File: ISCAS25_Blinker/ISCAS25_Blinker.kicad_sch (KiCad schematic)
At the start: 18 parts, among them J1 USB_C_Receptacle_PowerOnly_6P, Q1 BC846, Q2 BC857, U2 NE555D

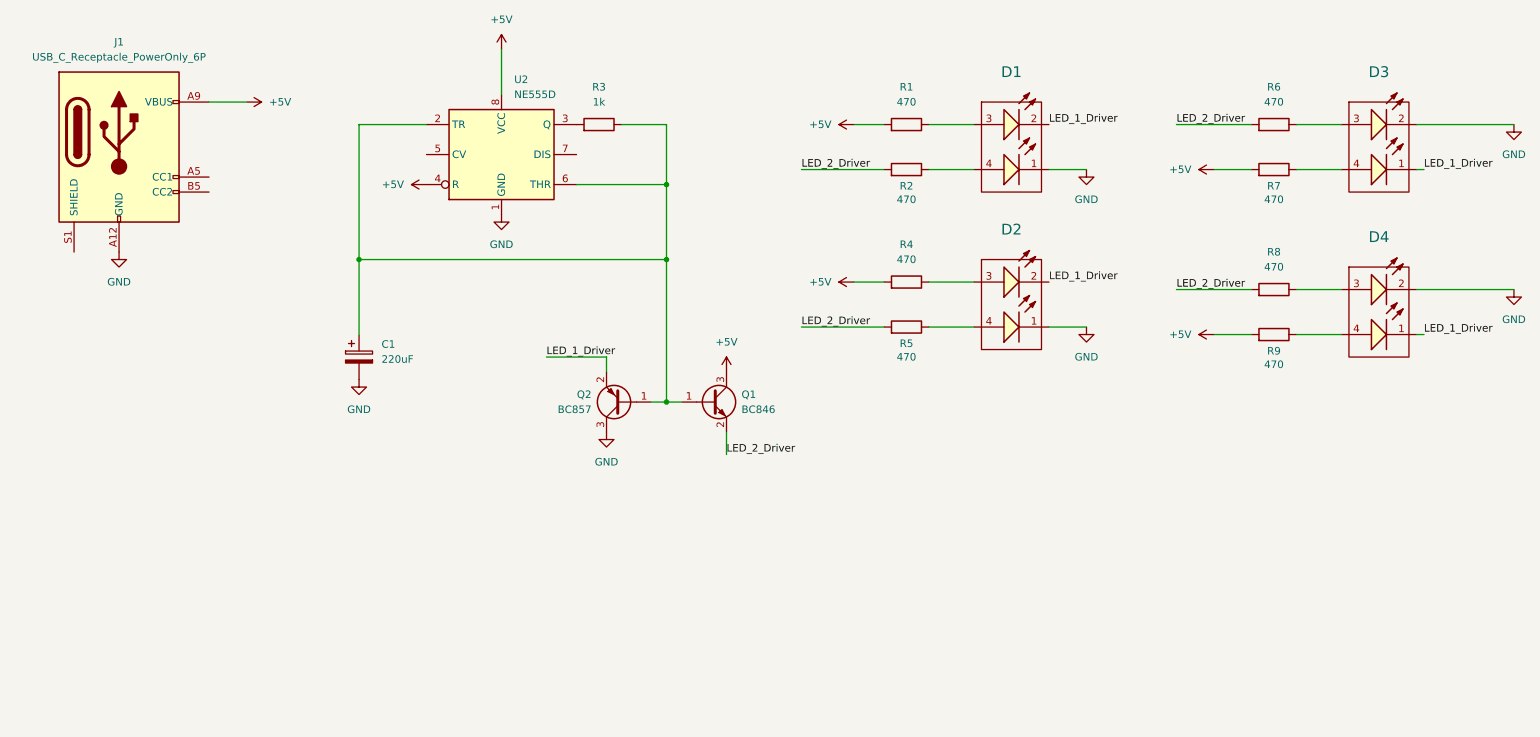
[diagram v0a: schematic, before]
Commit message: Finished but not panelized
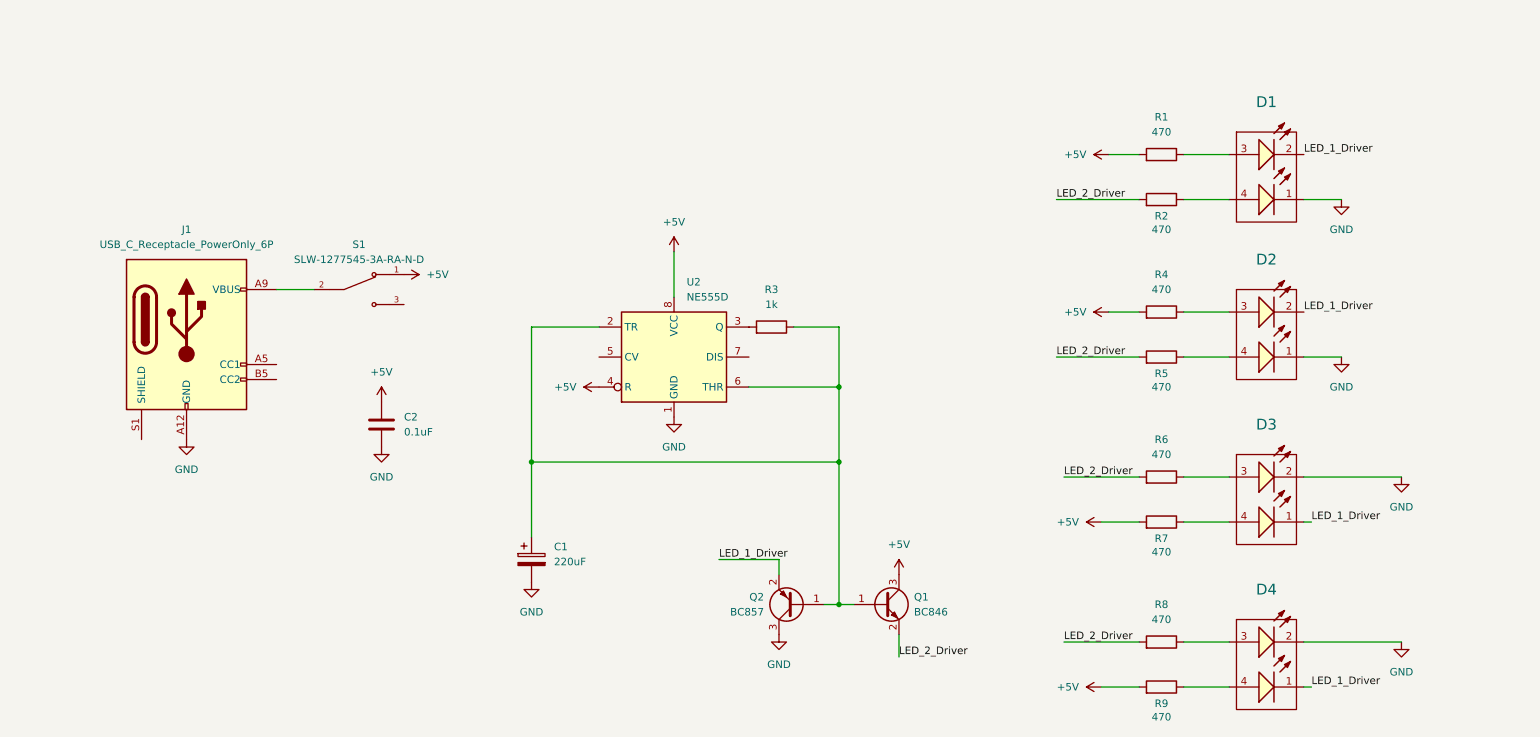
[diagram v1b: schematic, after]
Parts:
- added C2: 0.1uF, Capacitor_SMD:C_0603_1608Metric, symbol Device:C
- added S1: SLW-1277545-3A-RA-N-D, Library:SW_SLW-1277545-3A-RA-N-D, symbol Library:SLW-1277545-3A-RA-N-D
- C1: footprint Capacitor_THT:C_Rect_L11.0mm_W6.4mm_P10.00mm_MKT -> Capacitor_THT:CP_Radial_D6.3mm_P2.50mm
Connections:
- net +5V: now also C2.1, S1.1; no longer J1.A9 (VBUS), J1.B9 (VBUS)
- net GND: now also C2.2
- new net: J1.A9 (VBUS), J1.B9 (VBUS), S1.2
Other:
- moved on the sheet: C1, D1, D2, D3, D4, J1, Q1, Q2, R1, R2, R3, R4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
